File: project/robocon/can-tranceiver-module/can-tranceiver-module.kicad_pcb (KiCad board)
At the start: 2 copper layers, 26.5 x 33 mm, 12 parts, among them J1 Conn_01x07_Pin, SW1 SlideSwitch, U1 MCP2562-E-P, U2 AZ1117-3.3

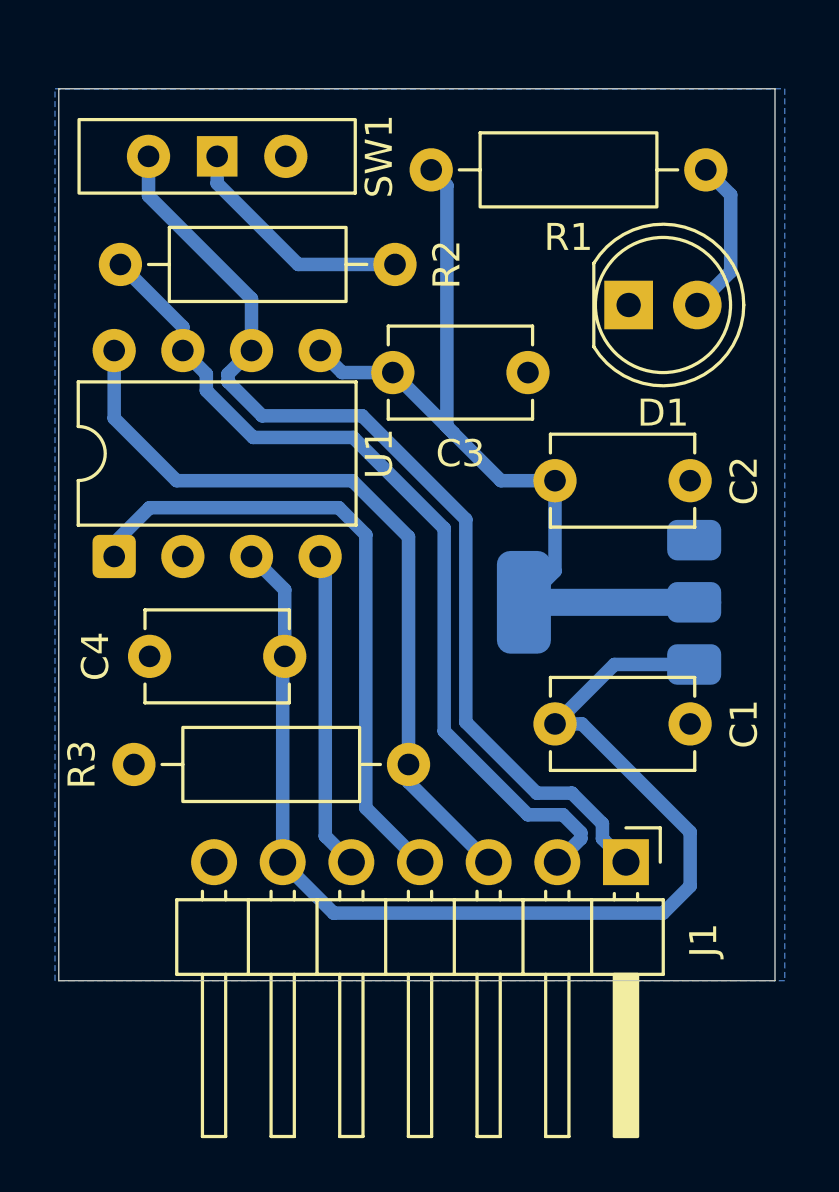
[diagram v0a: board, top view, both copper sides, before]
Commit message: 2026/03/23/21:25
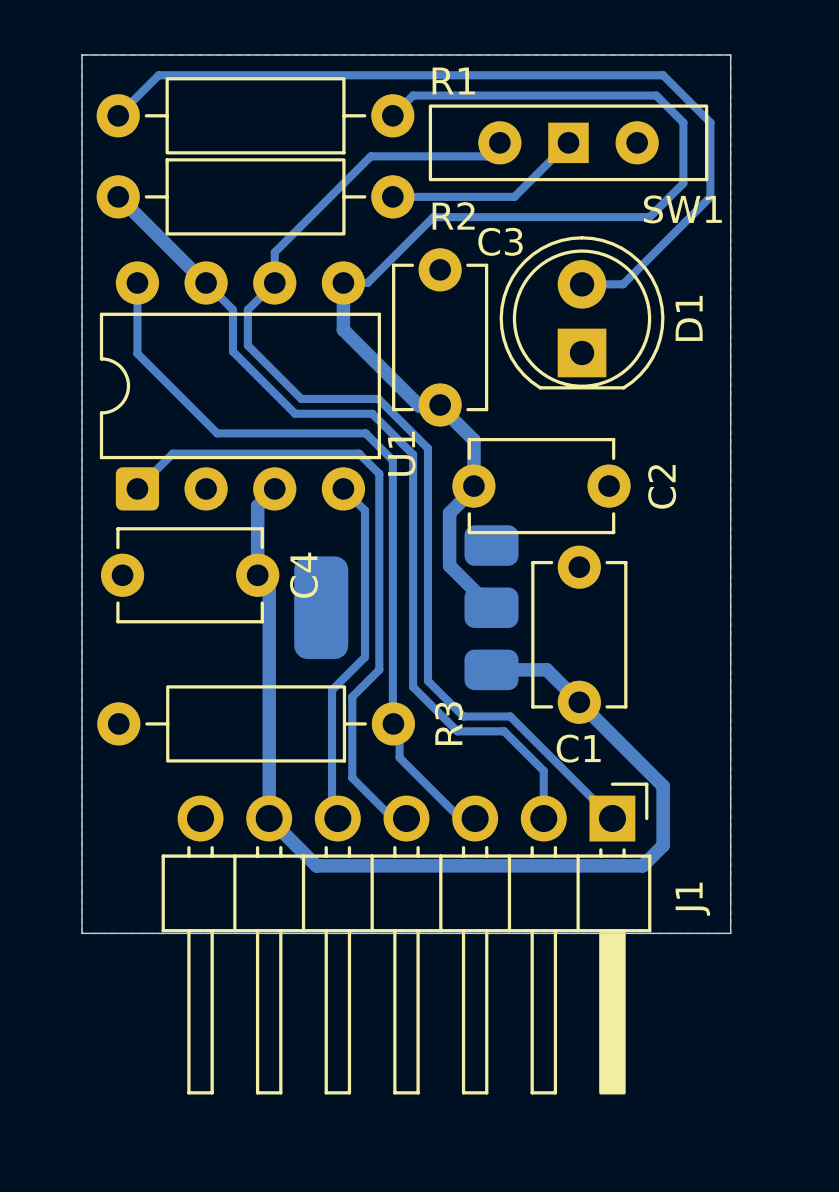
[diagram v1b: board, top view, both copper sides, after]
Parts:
- moved SW1 13.0 mm to (134.0, 53.0)
- moved U2 7.50 mm to (128.0, 70.2)
- moved C4 3.16 mm to (117.5, 69.0)
- moved C2 3.01 mm to (130.5, 65.7)
- moved U1 2.64 mm to (118.1, 65.8)
- moved R2 2.50 mm to (117.3, 55.0)
- moved D1 2.48 mm to (134.5, 60.8), turned to 90 degrees
- moved R1 2.45 mm to (127.5, 52.0), turned to 180 degrees
- moved C3 2.12 mm to (129.2, 62.7), turned to 90 degrees
- moved J1 1.69 mm to (135.6, 78.0)
- moved R3 1.60 mm to (127.5, 74.5)
- moved C1 1.20 mm to (134.4, 73.7), turned to 90 degrees
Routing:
- net Net-(D1-A): track 5.89 -> 32.1 mm
- net +3.3V: track 32.6 -> 43.3 mm
- net +5V: track 43.3 -> 38.6 mm
- net CAN-: track 37.1 -> 39.6 mm
- net Net-(SW1-B): track 8.82 -> 7.33 mm
- net RXD: track 11.8 -> 13.1 mm
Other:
- board size 26.5 x 33 mm -> 24 x 32.5 mm

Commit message: 2026/03/23/22:21
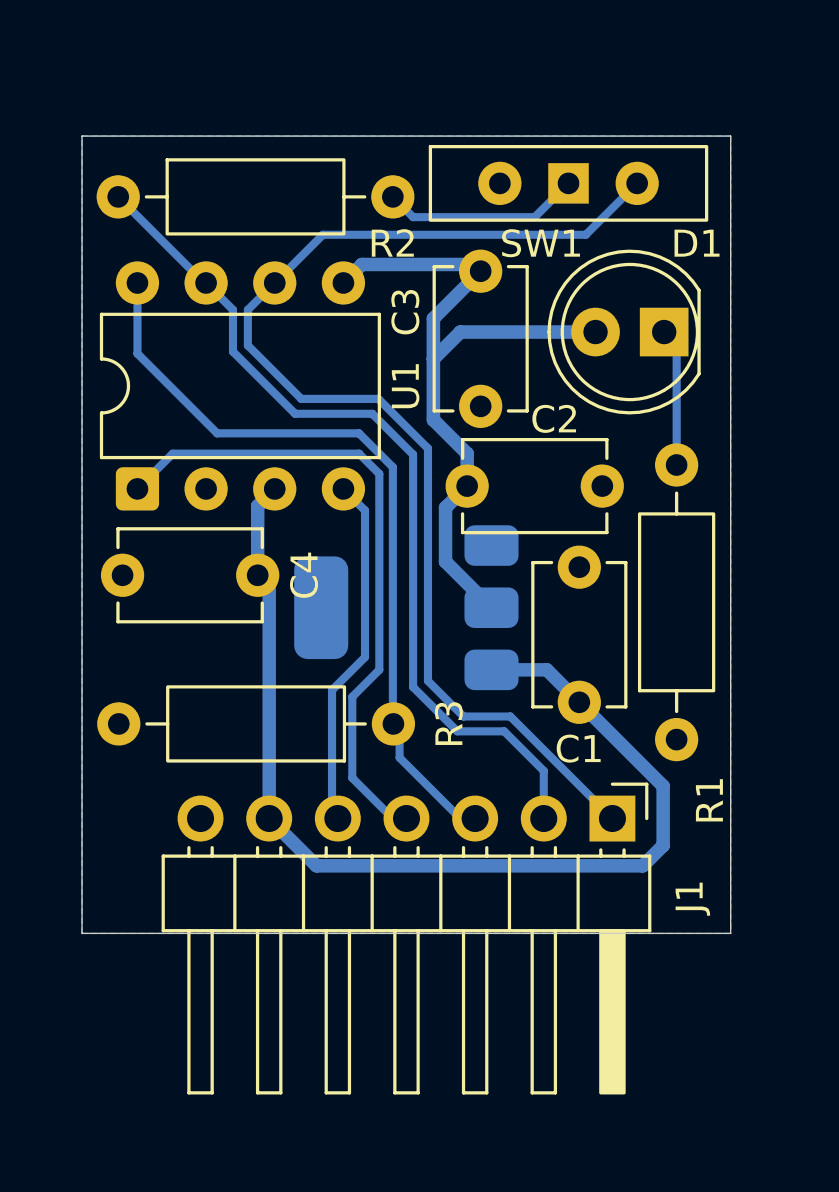
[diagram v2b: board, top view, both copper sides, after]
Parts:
- moved R1 25.4 mm to (138.0, 75.1), turned to 90 degrees
- moved C3 5.17 mm to (130.8, 57.8), turned to -90 degrees
- moved D1 3.14 mm to (137.5, 60.0), turned to 180 degrees
- moved SW1 1.50 mm to (134.0, 54.5), turned to 0 degrees
- moved C2 0.25 mm to (130.2, 65.7)
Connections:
- D1 pad 1: GND -> Net-(D1-K)
- D1 pad 2: Net-(D1-A) -> +3.3V
- R1 pad 1: +3.3V -> GND
- R1 pad 2: Net-(D1-A) -> Net-(D1-K)
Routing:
- net Net-(D1-A): track 32.1 -> 0.00 mm
- net +3.3V: track 43.3 -> 26.6 mm
- net Net-(D1-K): track 0.00 -> 5.11 mm
- net CAN-: track 39.6 -> 43.4 mm
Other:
- board size 24 x 32.5 mm -> 24 x 29.5 mm
